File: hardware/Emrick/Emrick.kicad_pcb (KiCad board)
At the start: 4 copper layers, 41.5 x 71.5 mm, 87 parts, among them J1 LED_STRIP_CONNECTOR, J2 UFL, J3 Conn_02x05_Odd_Even, J4 BATT_CONN, P1 USB_C_Plug_USB2.0, Q1 Q_NPN_DGS, Q2 Q_NPN_DGS, Q3 Q_NPN_DGS, SW1 SW_SPST, SW2 SW_MEC_5E (RESET), U1 74HCT541, U2 CC1310, U3 TPS63020, U4 CP2102N, U5 MX25R8035F, U6 BQ24072, Y1 24MHz, Y2 32.768kHz

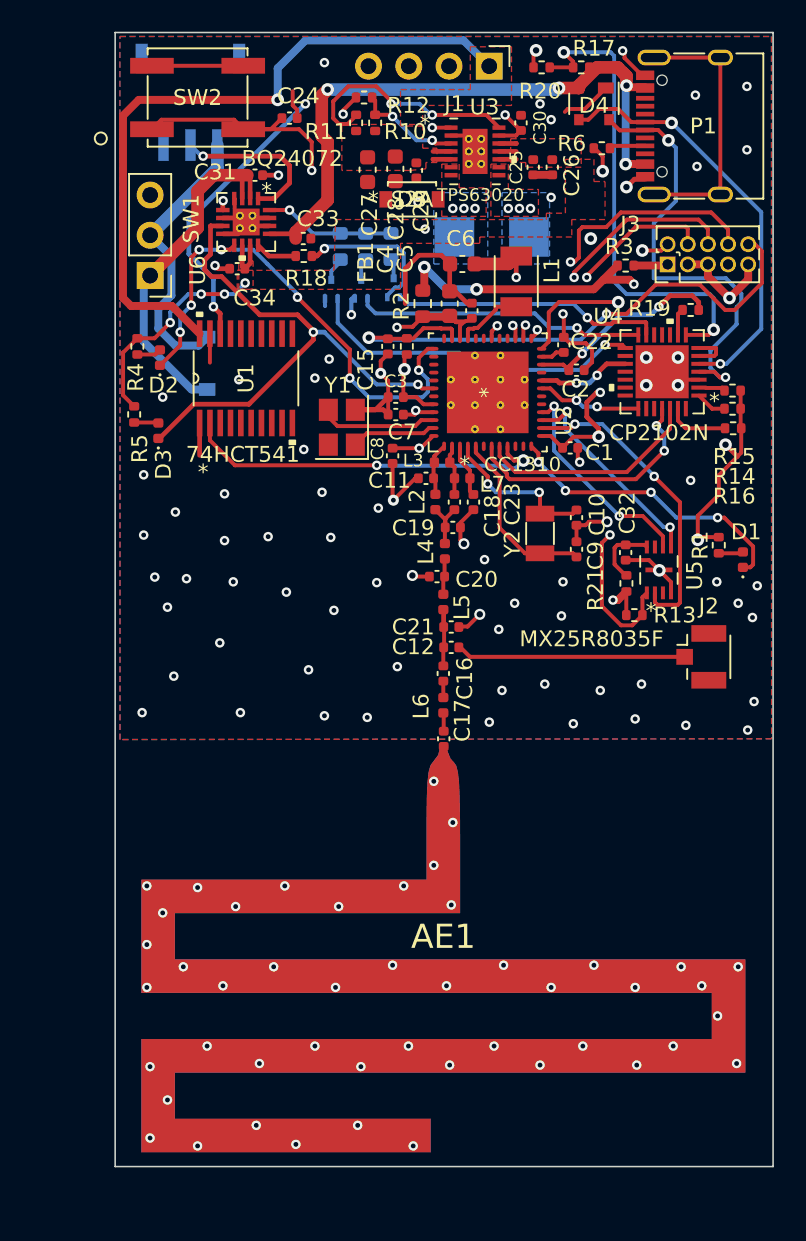
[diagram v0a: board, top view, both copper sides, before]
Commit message: some work on pcb and schematic
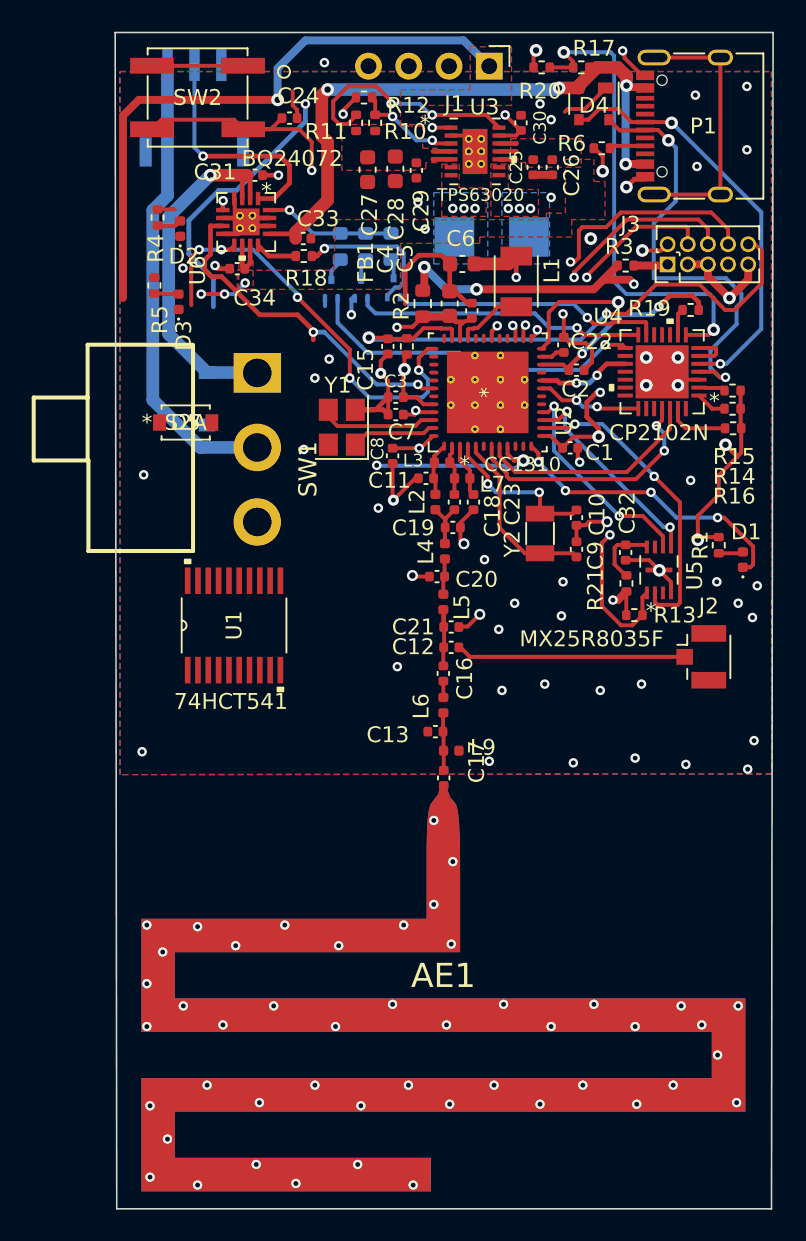
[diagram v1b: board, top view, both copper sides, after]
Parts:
- added C13: ?, Capacitor_SMD:C_0402_1005Metric, F.Cu at (101.9, 63.6)
- added L9: ?, Inductor_SMD:L_0402_1005Metric, F.Cu at (102.9, 64.8)
- C12: value 100pF -> ?
- SW1: footprint Connector_PinHeader_2.54mm:PinHeader_1x03_P2.54mm_Vertical -> switch:SW-TH_3P-P4.70_L11.1-W12.7
- moved D5 20.0 mm to (86.1, 44.1)
- moved U1 15.6 mm to (89.2, 56.9)
- moved SW1 12.8 mm to (90.7, 45.7), turned to -90 degrees
- moved D3 8.23 mm to (85.7, 36.5)
- moved R5 8.23 mm to (84.2, 35.5)
- moved D2 8.23 mm to (85.8, 31.9)
- moved R4 8.23 mm to (84.4, 31.2)
- moved AE1 2.47 mm to (102.4, 79.9)
- moved C17 2.47 mm to (102.4, 66.5)
- moved D5 2.23 mm to (87.5, 42.6), turned to -90 degrees
- moved J4 1.86 mm to (86.7, 25.0), turned to 180 degrees
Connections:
- C25 pad 2: VDDS -> VBAT
- C26 pad 2: VDDS -> VBAT
- D5 pad 2: Net-(J4-Pad3) -> Net-(D5-Pad2)
- J4 pad 3: Net-(J4-Pad3) -> Net-(D5-Pad2)
- SW1 pad 2: Net-(J4-Pad3) -> Net-(D5-Pad2)
- U3 pad 10: VDDS -> VBAT
- U3 pad 11: VDDS -> VBAT
- U3 pad 12: VDDS -> VBAT
- U4 pad 6: unconnected-(U4-Pad6) -> VDDS
- U4 pad 7: VDDS -> VBAT
- U6 pad 10: VDDS -> unconnected-(U6-Pad10)
- U6 pad 11: VDDS -> unconnected-(U6-Pad11)
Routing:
- net Net-(D5-Pad2): track 0.00 -> 29.3 mm
- net Net-(J4-Pad3): track 18.0 -> 0.00 mm
- net VDDS: track 125.2 -> 112.5 mm, vias 14 -> 13
- net BAT_PGOOD: track 34.1 -> 21.9 mm
- net LED_DATA_3V: track 23.5 -> 11.2 mm
- net BBReg_5V: track 46.7 -> 40.9 mm
- net BAT_TS: track 10.3 -> 15.3 mm
- net BAT_CHG: track 32.6 -> 28.0 mm, vias 7 -> 5
- net GND: track 108.6 -> 104.8 mm, vias 82 -> 61
- net VBAT: track 22.5 -> 26.0 mm, vias 0 -> 1
- net Net-(C13-Pad1): track 1.05 -> 3.45 mm
- net LED_DATA_5V: track 29.9 -> 28.7 mm, vias 2 -> 1
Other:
- board size 41.5 x 71.5 mm -> 41.5 x 74.2 mm
